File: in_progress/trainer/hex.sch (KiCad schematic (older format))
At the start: 31 parts

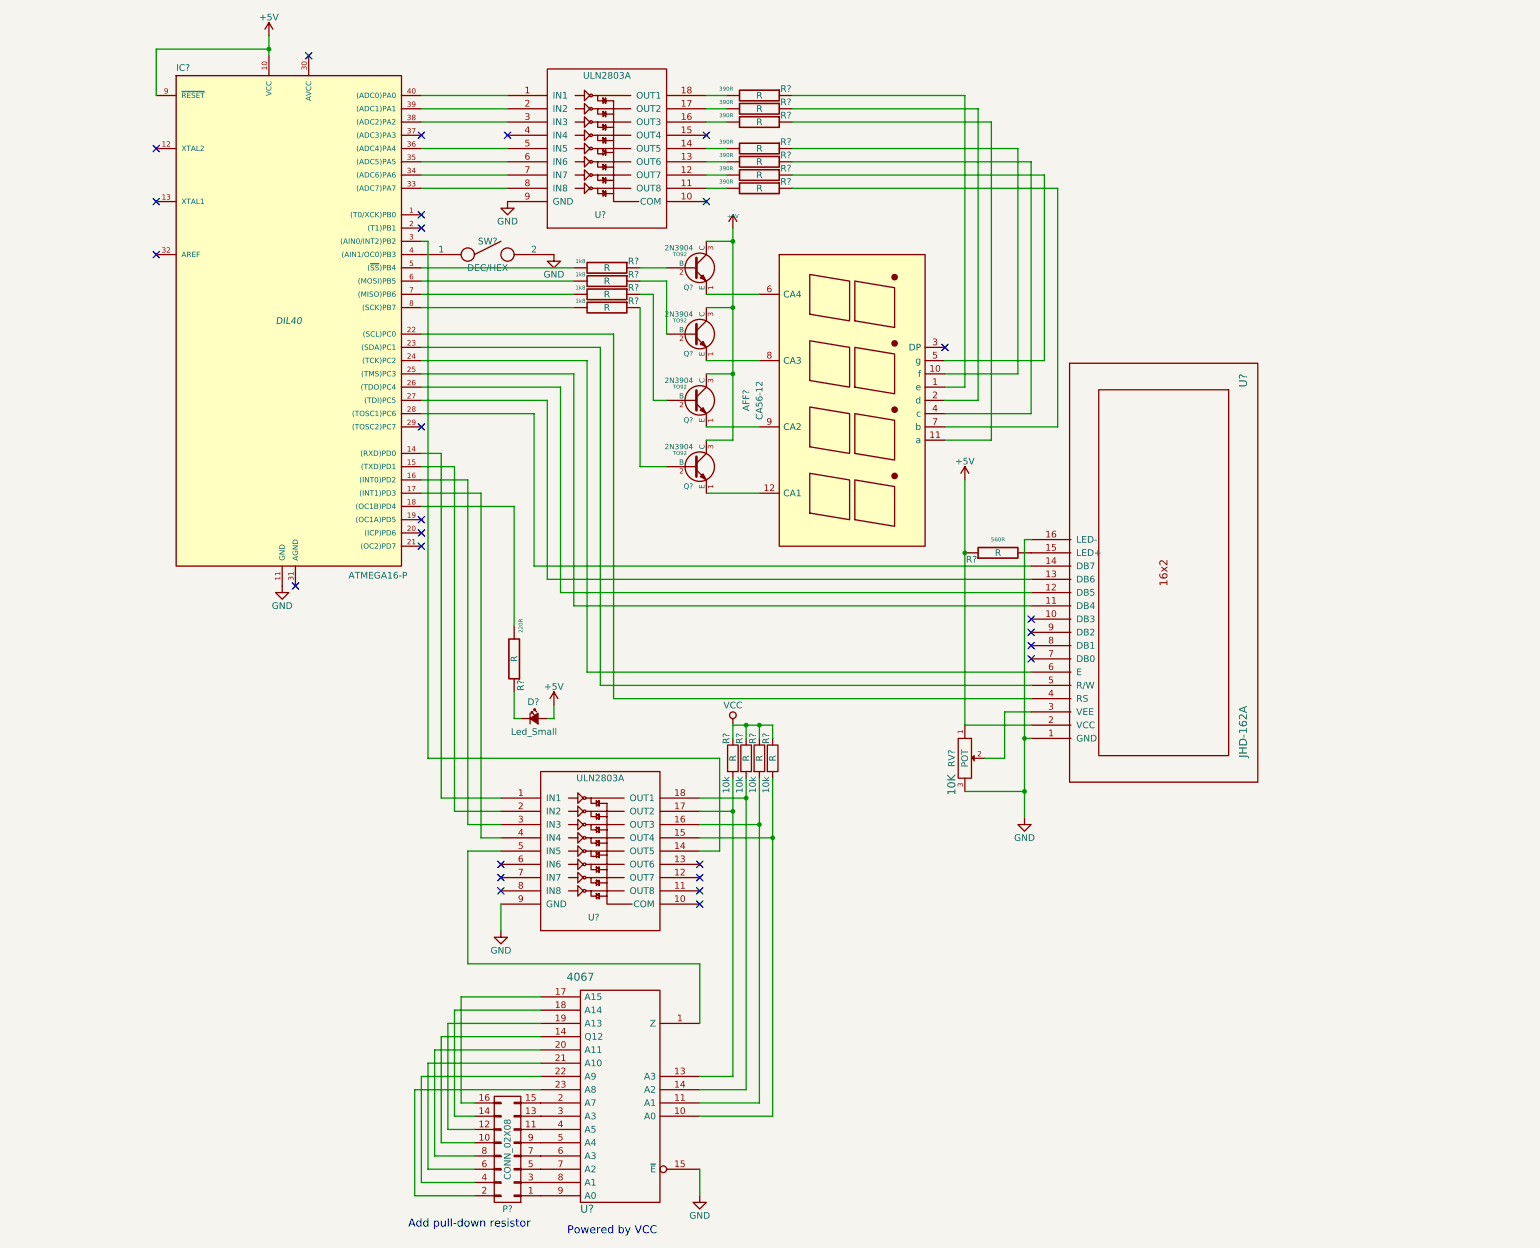
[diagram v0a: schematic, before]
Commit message: .
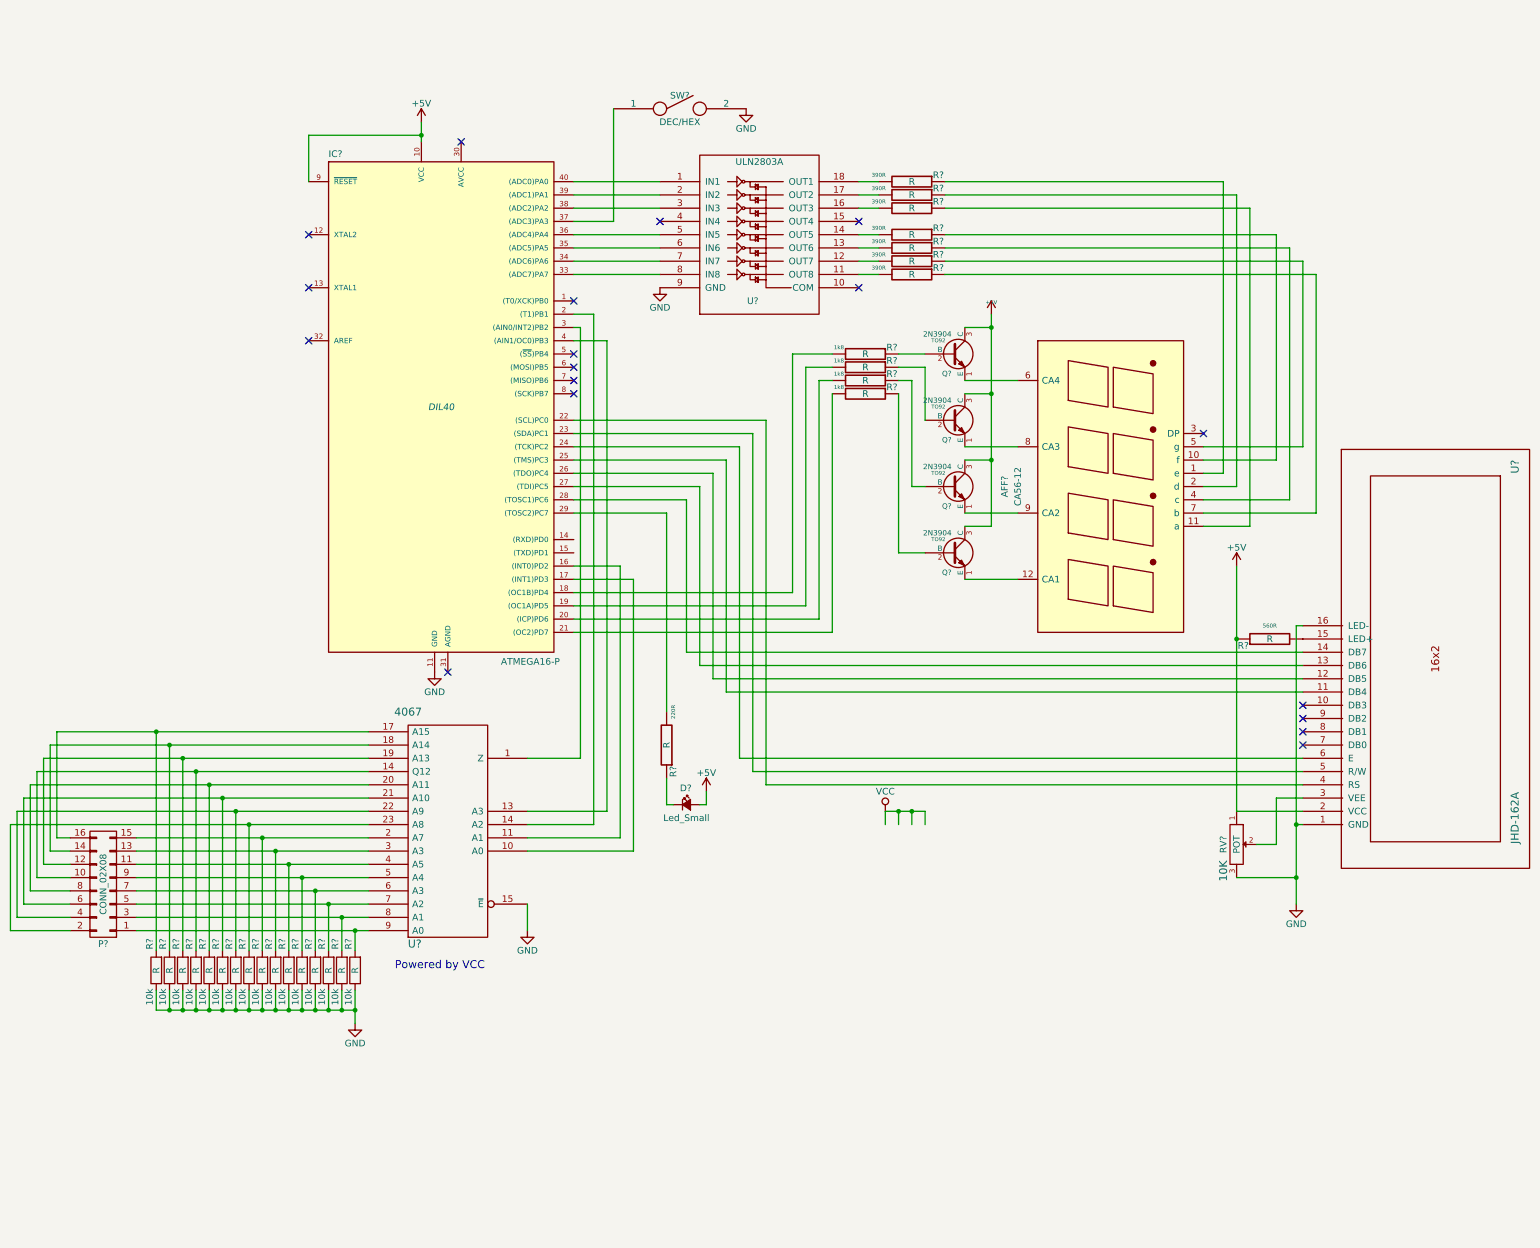
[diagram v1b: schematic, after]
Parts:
- removed R? (x4): R, 10k, symbol R
- removed U?: ULN2803A, symbol ULN2803A
- added R? (x16): R, 10k, symbol R
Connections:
- net GND: now also R?.1, R?.1, R?.1, R?.1, R?.1, R?.1, R?.1, R?.1, R?.1, R?.1, R?.1, R?.1, R?.1, R?.1, R?.1, R?.1
- net at U?.1 (Z): now also IC?.3 ((AIN0/INT2)PB2)
- net at U?.10 (A0): now also IC?.17 ((INT1)PD3)
- net at U?.11 (A1): now also IC?.16 ((INT0)PD2)
- net at U?.13 (A3): now also IC?.4 ((AIN1/OC0)PB3)
- net at P?.10 (P10), U?.14 (Q12): now also R?.2
- net at U?.14 (Q12): now also IC?.2 ((T1)PB1)
- net at P?.16 (P16), U?.17 (A15): now also R?.2
- net at P?.14 (P14), U?.18 (A14): now also R?.2
- net at P?.12 (P12), U?.19 (A13): now also R?.2
- net at P?.15 (P15), U?.2 (A7): now also R?.2
- net at P?.8 (P8), U?.20 (A11): now also R?.2
- net at P?.6 (P6), U?.21 (A10): now also R?.2
- net at P?.4 (P4), U?.22 (A9): now also R?.2
- net at P?.2 (P2), U?.23 (A8): now also R?.2
- net at P?.13 (P13), U?.3 (A3): now also R?.2
- net at P?.11 (P11), U?.4 (A5): now also R?.2
- net at P?.9 (P9), U?.5 (A4): now also R?.2
- net at P?.7 (P7), U?.6 (A3): now also R?.2
- net at P?.5 (P5), U?.7 (A2): now also R?.2
- net at P?.3 (P3), U?.8 (A1): now also R?.2
- net at P?.1 (P1), U?.9 (A0): now also R?.2
- net at R?.2: now also IC?.18 ((OC1B)PD4); no longer IC?.5 ((~SS~)PB4)
- net at R?.2: now also IC?.19 ((OC1A)PD5); no longer IC?.6 ((MOSI)PB5)
- net at R?.2: now also IC?.20 ((ICP)PD6); no longer IC?.7 ((MISO)PB6)
- net at R?.2: now also IC?.21 ((OC2)PD7); no longer IC?.8 ((SCK)PB7)
- net at R?.2: now also IC?.29 ((TOSC2)PC7); no longer IC?.18 ((OC1B)PD4)
- net at IC?.37 ((ADC3)PA3): now also SW?.1
- no-connect marks 27 -> 18
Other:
- note removed: "Add pull-down resistor"
- moved on the sheet: AFF?, D?, IC?, P?, Q?, R?, RV?, SW?, U?
